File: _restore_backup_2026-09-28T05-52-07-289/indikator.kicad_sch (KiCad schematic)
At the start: 104 parts, among them J1 Conn_01x02, Q1 AO3400A, Q10 AO3400A, Q11 AO3400A, Q12 AO3400A, Q13 AO3400A, Q14 AO3400A, Q15 AO3400A, Q16 AO3400A, Q17 AO3400A, Q18 AO3400A, Q19 AO3400A, Q2 AO3400A, Q20 AO3400A, Q21 AO3400A, Q22 AO3400A, Q23 AO3400A, Q24 AO3400A, Q3 AO3400A, Q4 AO3400A, Q5 AO3400A, Q6 AO3400A, Q7 AO3400A, Q8 AO3400A, Q9 AO3400A, U1 XIAO-ESP32-C3-SMD, U2 74HC595, U3 74HC595, U4 74HC595

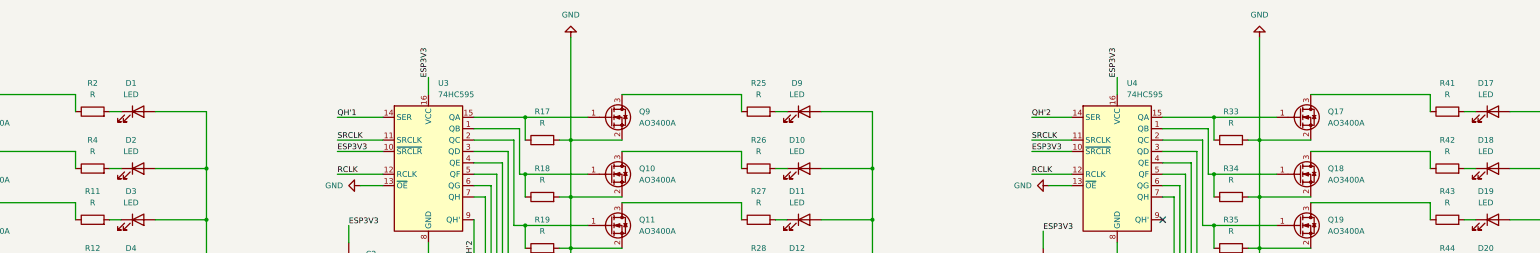
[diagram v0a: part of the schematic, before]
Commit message: ROUTING IS FRICKIN IMPOSSIBLE BRUH
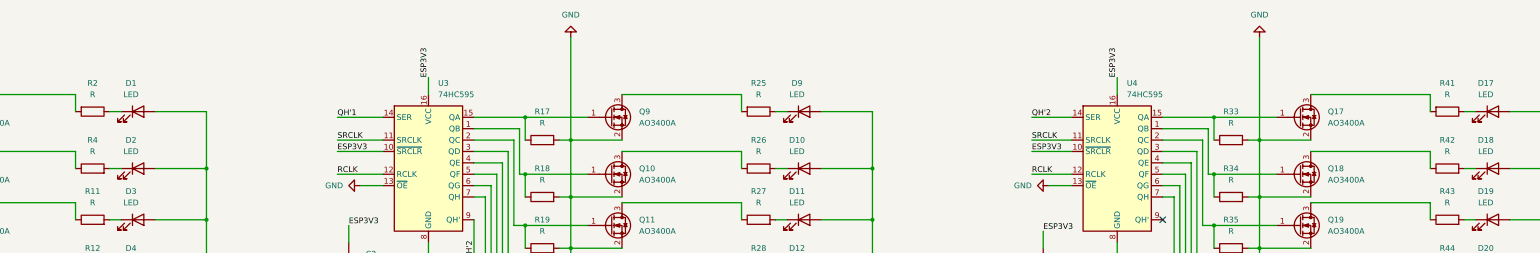
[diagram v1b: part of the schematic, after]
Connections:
- net at D1.1 (K): now also R2.1; no longer R2.2
- net at D9.1 (K): now also R25.1; no longer R25.2
- net at Q17.3 (D): now also R41.2; no longer R41.1
- net at D17.1 (K): now also R41.1; no longer R41.2
- net at Q9.3 (D): now also R25.2; no longer R25.1
- net at Q1.3 (D): now also R2.2; no longer R2.1
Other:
- moved on the sheet: R2, R25, R41
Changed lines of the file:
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@@
 	(symbol
 		(lib_id "Device:R")
-		(at 539.75 59.69 90)
+		(at 539.75 59.69 270)
 		(unit 1)
 		(body_style 1)
@@
 		)
 		(property "Footprint" "Resistor_SMD:R_0805_2012Metric"
-			(at 539.75 61.468 90)
+			(at 539.75 57.912 90)
 			(hide yes)
 			(show_name no)
@@
 	(symbol
 		(lib_id "Device:R")
-		(at 386.08 59.69 90)
+		(at 386.08 59.69 270)
 		(unit 1)
 		(body_style 1)
@@
 		)
 		(property "Footprint" "Resistor_SMD:R_0805_2012Metric"
-			(at 386.08 61.468 90)
+			(at 386.08 57.912 90)
 			(hide yes)
 			(show_name no)
@@
 	(symbol
 		(lib_id "Device:R")
-		(at 237.49 59.69 90)
+		(at 237.49 59.69 270)
 		(unit 1)
 		(body_style 1)
@@
 		)
 		(property "Footprint" "Resistor_SMD:R_0805_2012Metric"
-			(at 237.49 61.468 90)
-			(hide yes)
-			(show_name no)
+			(at 237.49 57.912 90)
+			(hide yes)
+			(show_name no)
